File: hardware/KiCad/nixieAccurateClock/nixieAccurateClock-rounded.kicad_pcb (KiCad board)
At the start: 4 copper layers, 152.4 x 101.6 mm, 103 parts, among them J1 Conn_01x02_Pin, J10 Conn_01x02_Pin, J17 Conn_02x05_Odd_Even, J2 Conn_01x02_Pin, J3 Conn_01x02_Pin, J4 pico iCE (A), J5 pico iCE (B), J6 Conn_01x02_Pin, J7 Conn_01x02_Pin, J8 Conn_Coaxial, J9 Conn_01x02_Pin, Q1 PZTA42, Q2 PZTA42, Q3 PZTA42, Q4 PZTA42, Q5 PZTA42, Q6 PZTA42, SW1 SW_DIP_x08, U1 MCP23008-xSO, U2 LTR-329ALS-01, U3 PX1125T, U6 ADC0820BCWMX

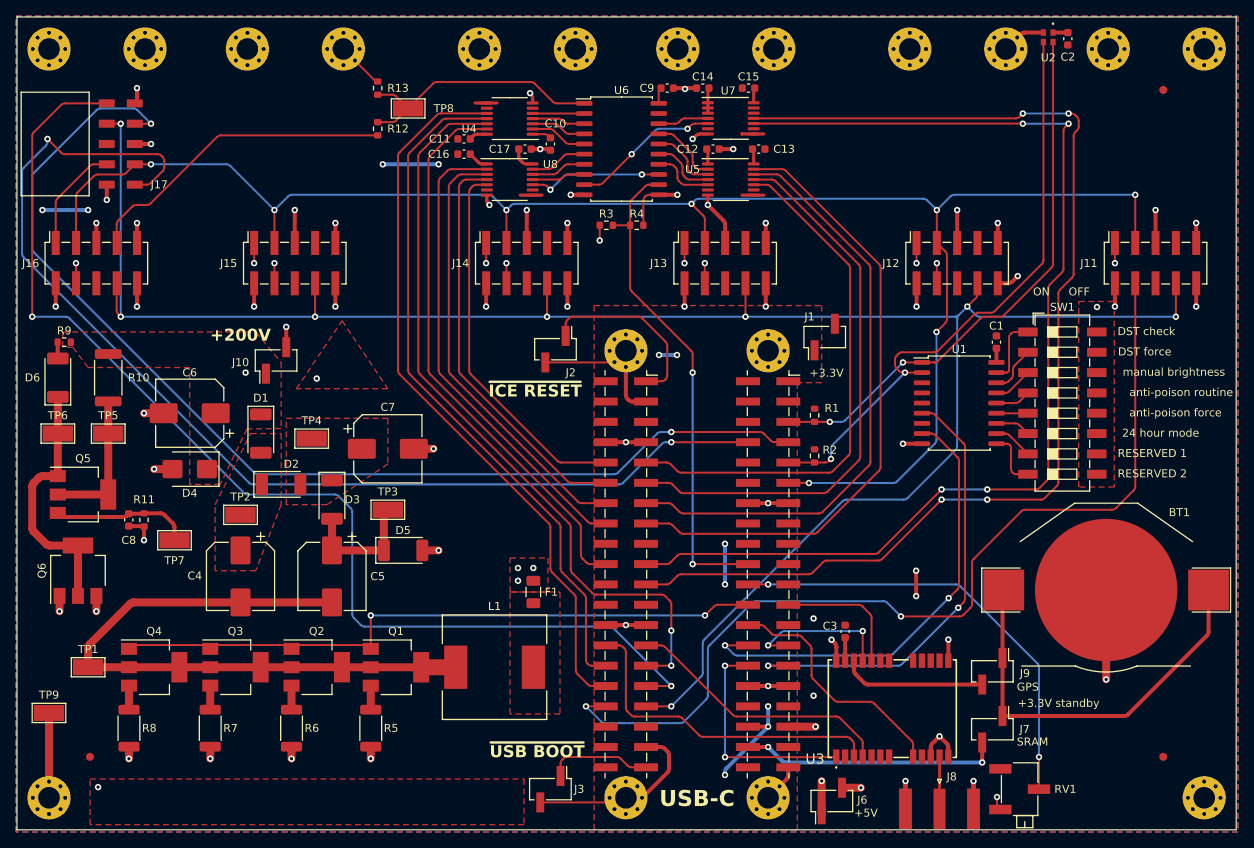
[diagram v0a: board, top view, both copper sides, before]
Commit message: Clean up clearances
Set board clearances, add dimension annotations, clean up pour dimensions
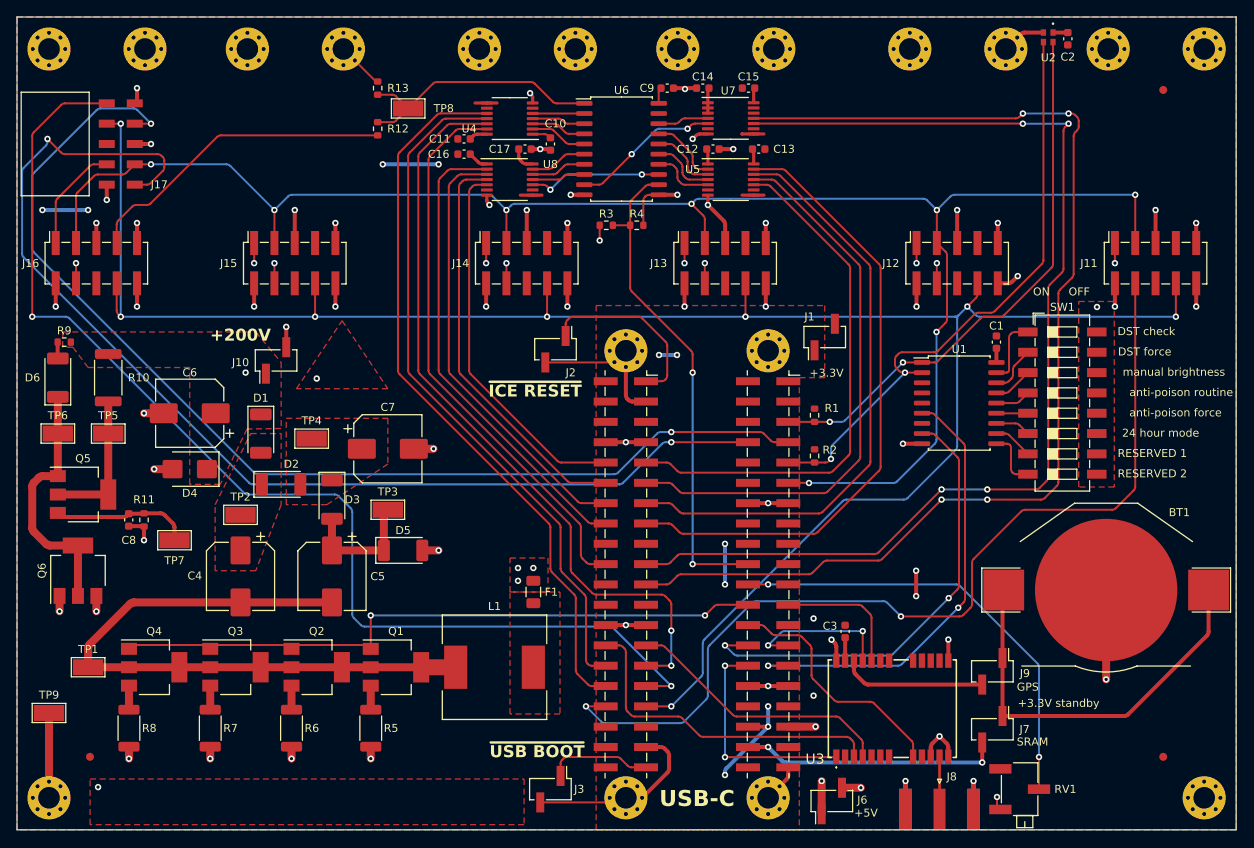
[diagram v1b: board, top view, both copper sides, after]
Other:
- board text added: "0.2000 mm / 0.2000 mm"
- board text removed: "0.0000 mm / 0.0000 mm"

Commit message: Switch to 2.4 mm stackup
PCBWAY001 is cheaper than PCBWAY209 (2 oz copper) for 0.2 mm prepreg (200 V clearance)
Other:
- board text added: "0.035 mm"
- board text added: "0.196 mm"
- board text added: "0.2500 mm / 0.2500 mm"
- board text added: "1.9 mm"
- board text added: "2.4520 mm"
- board text added: "Dielectric"
- board text removed: "0.0525 mm"
- board text removed: "0.07 mm"
- board text removed: "0.2000 mm / 0.2000 mm"
- board text removed: "0.22 mm"
- board text removed: "0.895 mm"
- board text removed: "1.6000 mm"
- board text removed: "Dielectric 1"
- board text removed: "Dielectric 2"
- board text removed: "Dielectric 3"

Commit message: Switch to stackup PCBWAY206
2.4 mm board is incompatible with SMA connector
Clean up outdated board notes
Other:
- board text added: "1.1 mm"
- board text added: "1.6520 mm"
- board text added: "Dielectric 1"
- board text added: "Dielectric 2"
- board text added: "Dielectric 3"
- board text added: "Epoxy"
- board text removed: "1.9 mm"
- board text removed: "2.4520 mm"
- board text removed: "Dielectric"
